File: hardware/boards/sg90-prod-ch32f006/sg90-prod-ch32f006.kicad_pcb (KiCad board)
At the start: 4 copper layers, 12.5 x 10 mm, 21 parts, among them J1 Servo Input, J2 Debug, J3 Motor, J4 Potentiometer, Q1 BRCS150P02ZJ, U1 CH32V006F8U6, U2 DRV8837C, U3 74LVC1G07

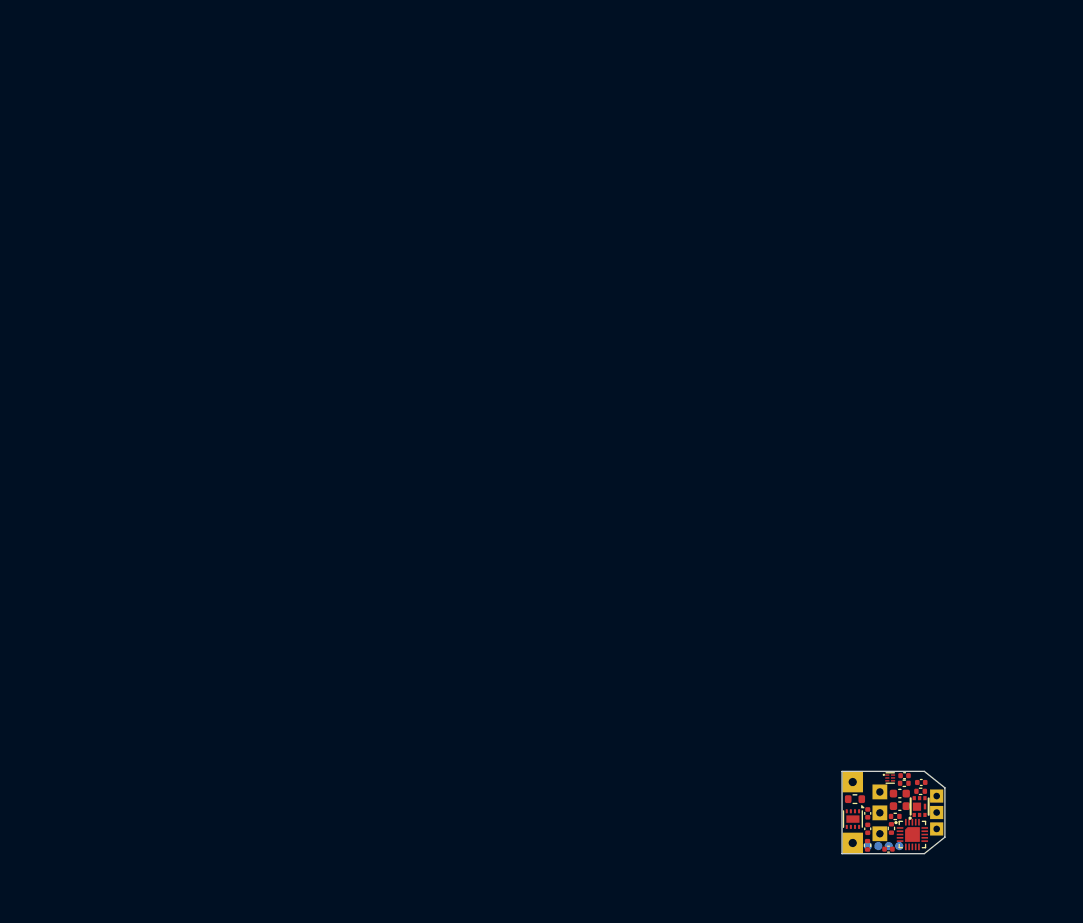
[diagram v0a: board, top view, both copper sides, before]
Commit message: re-organize shared folders
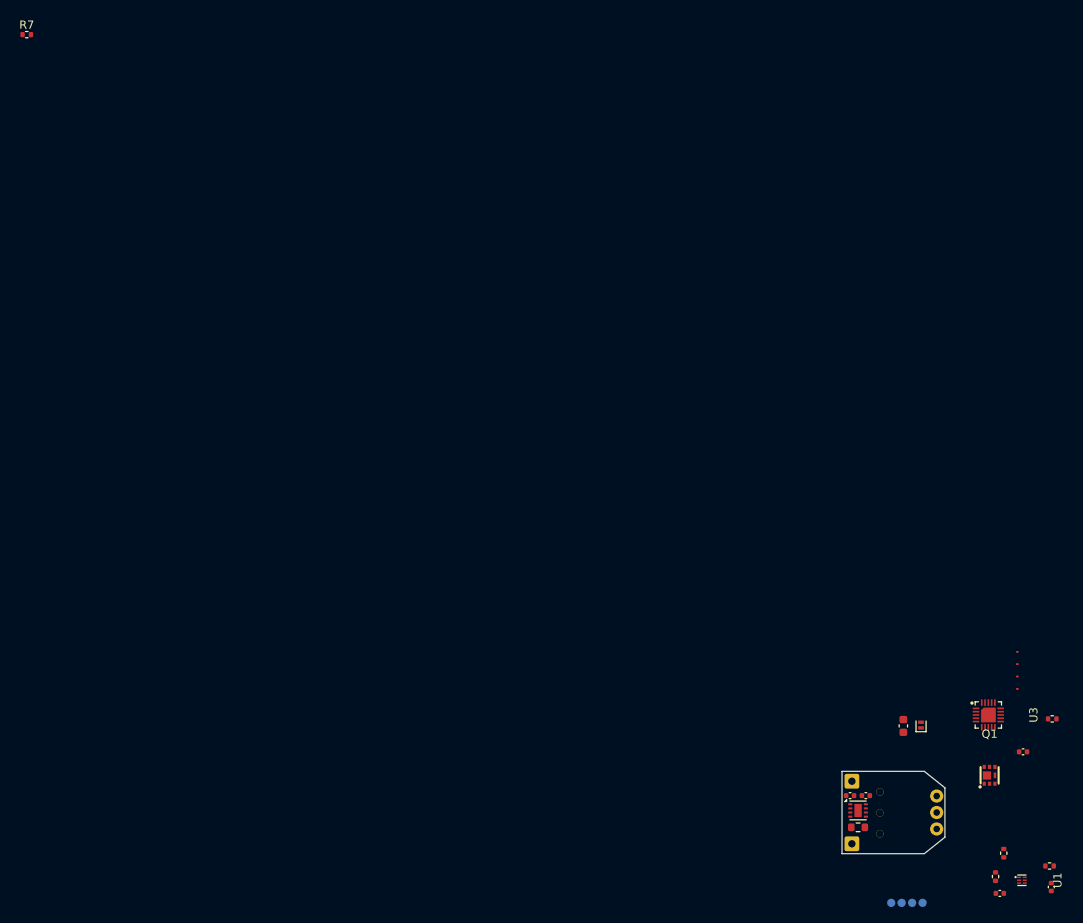
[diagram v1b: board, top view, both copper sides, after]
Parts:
- removed C7: 10µF, Capacitor_SMD:C_0603_1608Metric
- removed R9: 1kΩ, Resistor_SMD:R_0402_1005Metric
- added D1: PESD5V0L1UL, Diode_SMD:D_SOD-882, F.Cu at (109.6, 84.4)
- added NT1: NetTie_2, shared:NetTie-2_SMD_0.2mm, F.Cu at (121.3, 75.5)
- added NT2: NetTie_2, shared:NetTie-2_SMD_0.2mm, F.Cu at (121.3, 77.0)
- added NT3: NetTie_2, shared:NetTie-2_SMD_0.2mm, F.Cu at (121.3, 78.5)
- added NT4: NetTie_2, shared:NetTie-2_SMD_0.2mm, F.Cu at (121.3, 80.0)
- added R7: 10kΩ, Resistor_SMD:R_0402_1005Metric, F.Cu at (0.95, 0.49)
- C1: value 0.1µF -> 10µF; footprint Capacitor_SMD:C_0402_1005Metric -> Capacitor_SMD:C_0603_1608Metric
- C2: value 47nF -> 0.1µF
- C6: value 10µF -> 47nF; footprint Capacitor_SMD:C_0603_1608Metric -> Capacitor_SMD:C_0402_1005Metric
- J1: footprint common:Servo_Output_Pads -> shared:Servo_Output_Pads; moved to B.Cu
- J2: footprint common:Debug_Pads_1x4_P1.27mm -> shared:Debug_Pads_1x4_P1.27mm
- J3: footprint common:Motor_Wire_Pads -> shared:Motor_Wire_Pads; moved to B.Cu
- J4: footprint common:Pot_Wire_Pads -> shared:Pot_Wire_Pads; moved to B.Cu
- Q1: footprint common:DFN-6L_L2.0-W2.0-P0.65-BL_BRCS300PXX -> shared:DFN-6L_L2.0-W2.0-P0.65-BL_BRCS300PXX
- R2: value 0.1Ω 1% -> 1kΩ; footprint Resistor_SMD:R_0603_1608Metric -> Resistor_SMD:R_0402_1005Metric
- R4: value 10kΩ -> 0.1Ω 1%; footprint Resistor_SMD:R_0402_1005Metric -> Resistor_SMD:R_0603_1608Metric
- U1: value CH32V006F8U6 -> 74LVC1G07; footprint common:UQFN-20_L3.0-W3.0-P0.40-BL-EP1.7 -> shared:TDFN-6_L1.0-W1.0-P0.35-BL
- U3: value 74LVC1G07 -> CH32V006F8U6; footprint common:TDFN-6_L1.0-W1.0-P0.35-BL -> shared:UQFN-20_L3.0-W3.0-P0.40-BL-EP1.7
- moved R2 25.9 mm to (125.5, 83.6)
- moved C2 20.3 mm to (125.4, 104.0), turned to -90 degrees
- moved C5 18.4 mm to (119.2, 104.8)
- moved R5 18.1 mm to (125.2, 101.5)
- moved R3 16.6 mm to (119.7, 99.9)
- moved C6 15.8 mm to (122.0, 87.6)
- moved C1 15.1 mm to (107.5, 84.5), turned to -90 degrees
- moved U1 14.4 mm to (121.8, 103.2)
- moved U3 14.2 mm to (117.8, 83.2)
- moved R1 13.9 mm to (118.7, 102.8)
- moved Q1 9.31 mm to (117.9, 90.5)
- moved J2 7.46 mm to (107.9, 106.0)
- moved R4 4.71 mm to (102.0, 96.8)
- moved C3 4.57 mm to (101.0, 93.0), turned to 180 degrees
- moved C4 2.17 mm to (102.9, 93.0), turned to 0 degrees
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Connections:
- C2 pad 1: /SEN_POT -> +5V
- C6 pad 1: +5V -> /SEN_POT
- J3 pad 1: /MOT_B -> /MOT_A
- J3 pad 2: /MOT_A -> /MOT_B
- J4 pad 3: /V_MCU -> +5V
- R1 pad 1: /nRST -> Net-(Q1-G)
- R2 pad 1: /GND_MOT -> +5V
- R2 pad 2: GND -> /DATA
- R4 pad 1: Net-(Q1-G) -> GND
- R4 pad 2: GND -> /GND_MOT
- U1 pad 1: /nRST -> unconnected-(U1-NC-Pad1)
- U1 pad 2: /GND_MOT -> /UART_TX
- U1 pad 3: /GND_MOT -> GND
- U1 pad 4: GND -> /DATA
- U3 pad 1: unconnected-(U3-NC-Pad1) -> /nRST
- U3 pad 2: /UART_TX -> /SEN_I
- U3 pad 3: GND -> /SEN_I
- U3 pad 4: /DATA -> GND
